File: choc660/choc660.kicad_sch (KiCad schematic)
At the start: 144 parts, among them SW1 SW_Push, SW10 SW_Push, SW11 SW_Push, SW12 SW_Push, SW13 SW_Push, SW14 SW_Push, SW15 SW_Push, SW16 SW_Push, SW17 SW_Push, SW18 SW_Push, SW19 SW_Push, SW2 SW_Push, SW20 SW_Push, SW21 SW_Push, SW22 SW_Push, SW23 SW_Push, SW24 SW_Push, SW25 SW_Push, SW26 SW_Push, SW27 SW_Push, SW28 SW_Push, SW29 SW_Push, SW3 SW_Push, SW30 SW_Push, SW31 SW_Push, SW32 SW_Push, SW33 SW_Push, SW34 SW_Push, SW35 SW_Push, SW36 SW_Push, SW37 SW_Push, SW38 SW_Push, SW39 SW_Push, SW4 SW_Push, SW40 SW_Push, SW41 SW_Push, SW42 SW_Push, SW43 SW_Push, SW44 SW_Push, SW45 SW_Push, SW46 SW_Push, SW47 SW_Push, SW48 SW_Push, SW49 SW_Push, SW5 SW_Push, SW50 SW_Push, SW51 SW_Push, SW52 SW_Push, SW53 SW_Push, SW54 SW_Push, SW55 SW_Push, SW56 SW_Push, SW57 SW_Push, SW58 SW_Push, SW59 SW_Push, SW6 SW_Push, SW60 SW_Push, SW61 SW_Push, SW62 SW_Push, SW63 SW_Push, SW64 SW_Push, SW65 SW_Push, SW66 SW_Push, SW67 SW_Push, SW68 SW_Push, SW7 SW_Push, SW8 SW_Push, SW9 SW_Push, U1 Elite-C

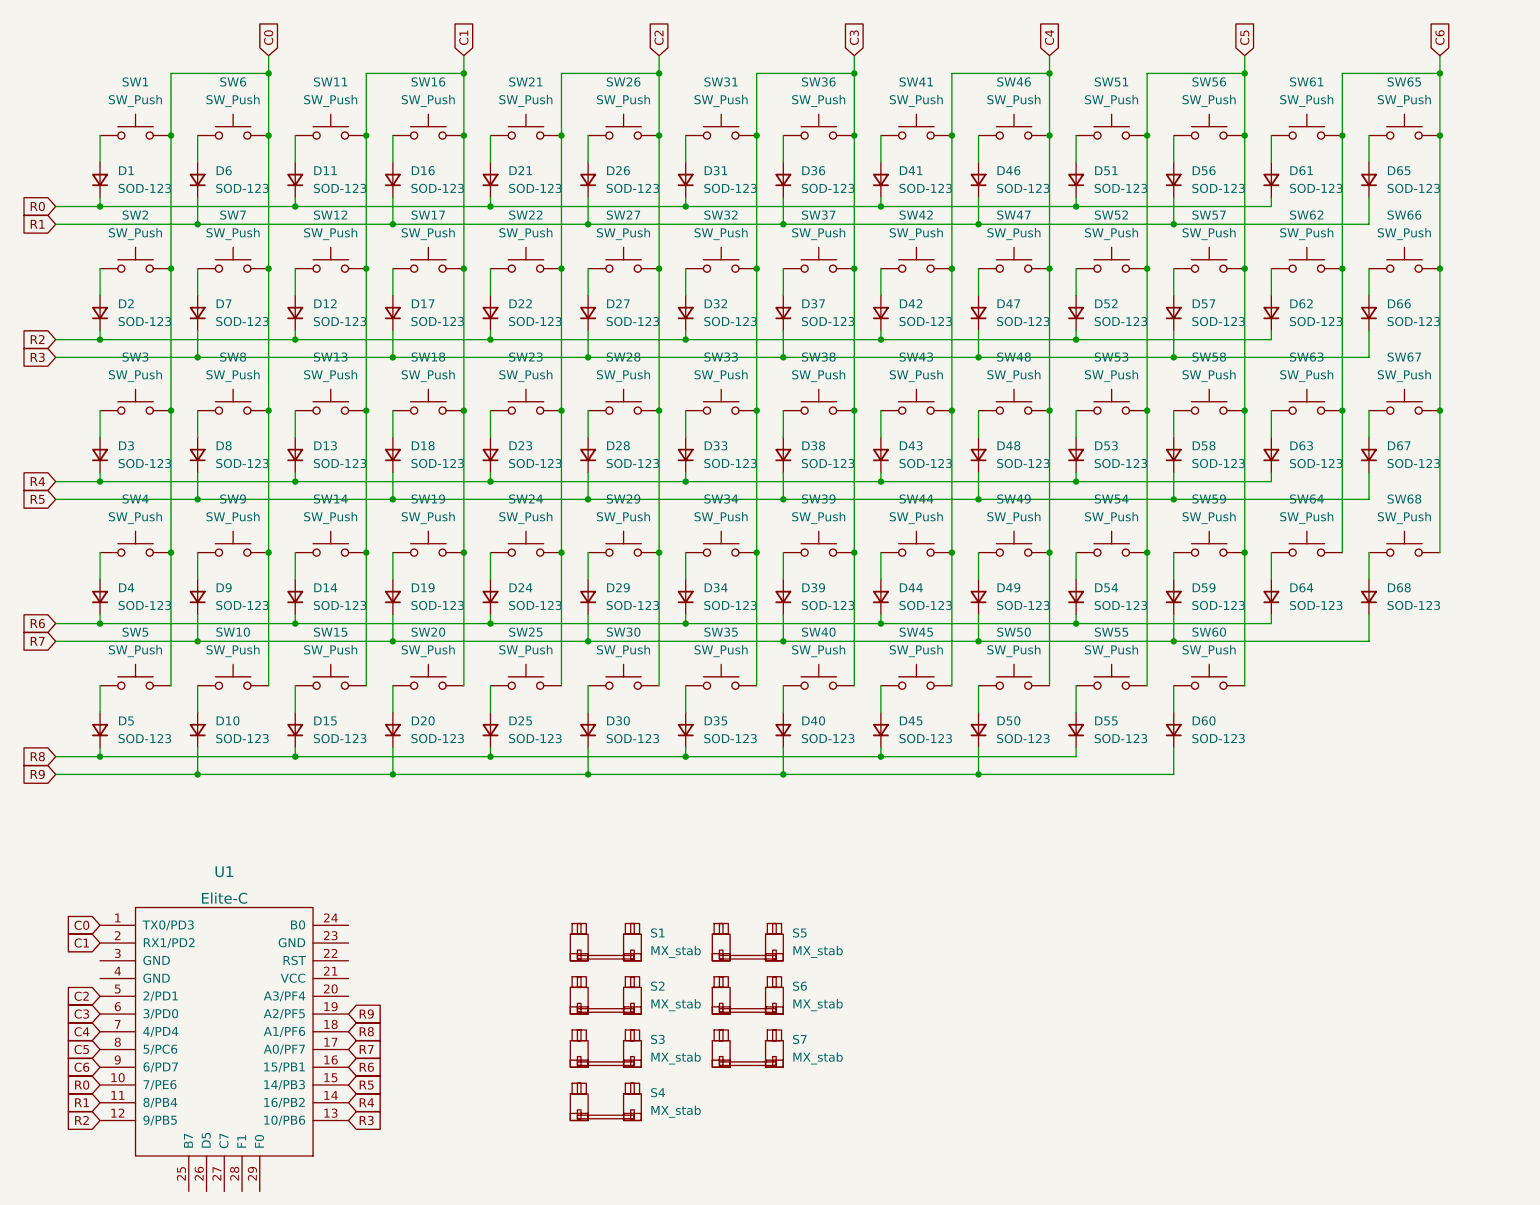
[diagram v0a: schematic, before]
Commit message: draw the rest of the owl?
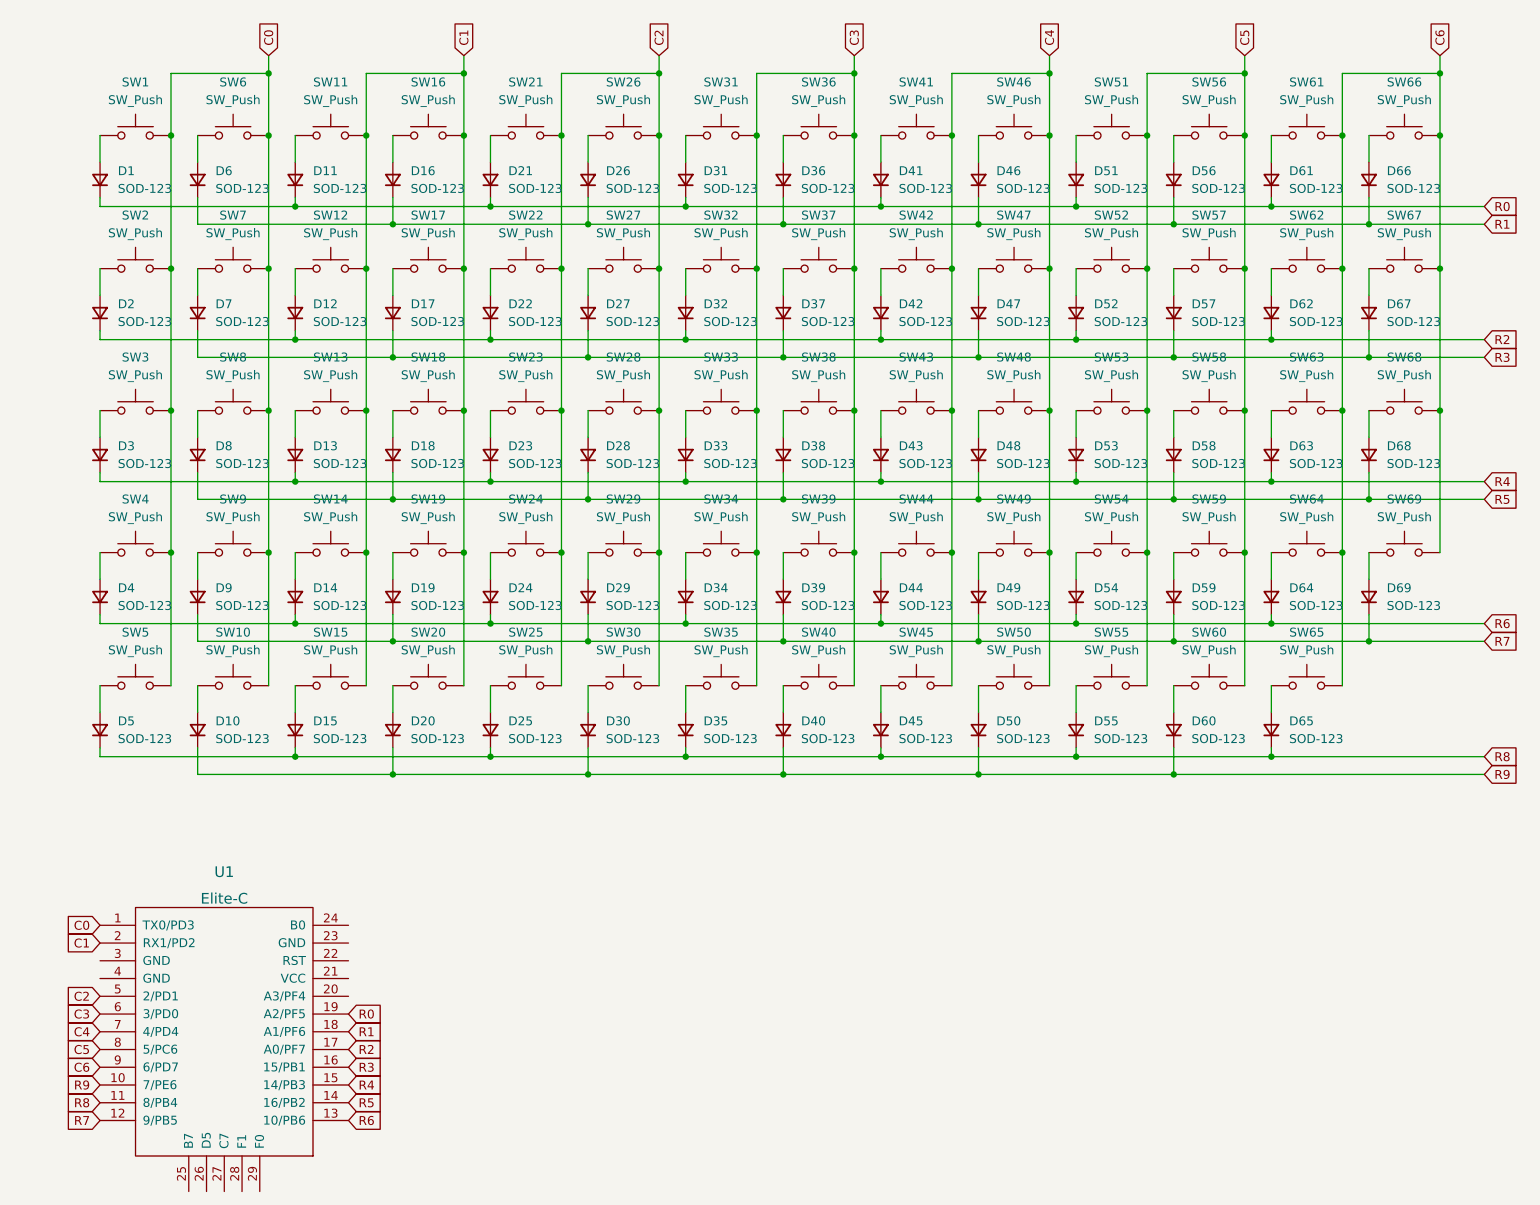
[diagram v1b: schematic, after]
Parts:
- removed S1, S2, S3, S4, S5, S6, S7: MX_stab, marbastlib-choc:STAB_choc_2u, symbol marbastlib-mx:MX_stab
- added D65: SOD-123, Diode_SMD:D_SOD-123, symbol Device:D_Small
- added SW65: SW_Push, marbastlib-choc:SW_choc_HS_1u, symbol Switch:SW_Push
- SW20, SW25, SW30, SW35, SW4, SW59, SW63: footprint marbastlib-choc:SW_choc_HS_1u -> marbastlib-choc:SW_choc_HS_1.5u
- SW66: renamed from SW65; footprint marbastlib-choc:SW_choc_HS_1u -> marbastlib-choc:SW_choc_HS_1.5u
- SW67: renamed from SW66; footprint marbastlib-choc:SW_choc_HS_1.5u -> marbastlib-choc:SW_choc_HS_1u
- renumbered D65 to D66, D66 to D67, D67 to D68, D68 to D69, SW67 to SW68, SW68 to SW69
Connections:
- net C6: now also SW65.2
- net R0: now also U1.19 (A2/PF5); no longer U1.10 (7/PE6)
- net R1: now also U1.18 (A1/PF6); no longer U1.11 (8/PB4)
- net R2: now also U1.17 (A0/PF7); no longer U1.12 (9/PB5)
- net R3: now also U1.16 (15/PB1); no longer U1.13 (10/PB6)
- net R4: now also U1.15 (14/PB3); no longer U1.14 (16/PB2)
- net R5: now also U1.14 (16/PB2); no longer U1.15 (14/PB3)
- net R6: now also U1.13 (10/PB6); no longer U1.16 (15/PB1)
- net R7: now also U1.12 (9/PB5); no longer U1.17 (A0/PF7)
- net R8: now also U1.11 (8/PB4), D65.1 (K); no longer U1.18 (A1/PF6)
- net R9: now also U1.10 (7/PE6); no longer U1.19 (A2/PF5)
- new net: D65.2 (A), SW65.1

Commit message: use non-hotswap footprints, also i made this backwards
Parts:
- SW1, SW10, SW11, SW12, SW13, SW14, SW15, SW16, SW17, SW18, SW19, SW21, SW22, SW23, SW24, SW26, SW27, SW28, SW29, SW31, SW32, SW33, SW34, SW36, SW37, SW38, SW39, SW40, SW41, SW42, SW43, SW44, SW45, SW46, SW47, SW48, SW49, SW5, SW50, SW51, SW52, SW53, SW54, SW55, SW56, SW57, SW58, SW6, SW60, SW61, SW62, SW64, SW65, SW67, SW68, SW69, SW7, SW8, SW9: footprint marbastlib-choc:SW_choc_HS_1u -> marbastlib-choc:SW_choc_1u
- SW2, SW25, SW3, SW30, SW35, SW4, SW59, SW63, SW66: footprint marbastlib-choc:SW_choc_HS_1.5u -> marbastlib-choc:SW_choc_1.5u
- SW20: footprint marbastlib-choc:SW_choc_HS_1.5u -> marbastlib-choc:SW_choc_1.25u

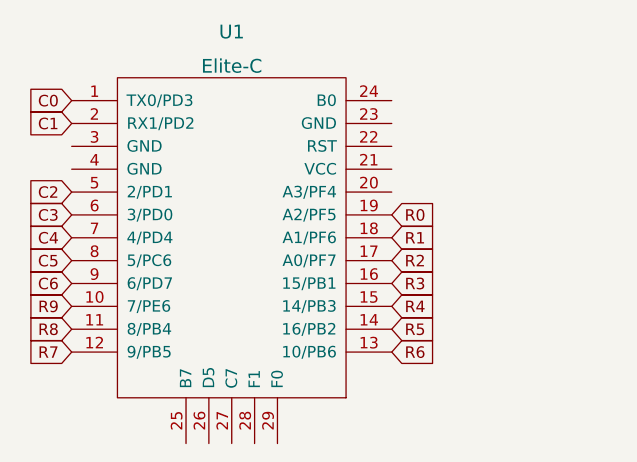
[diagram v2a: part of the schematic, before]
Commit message: retrace, reorient, and all that
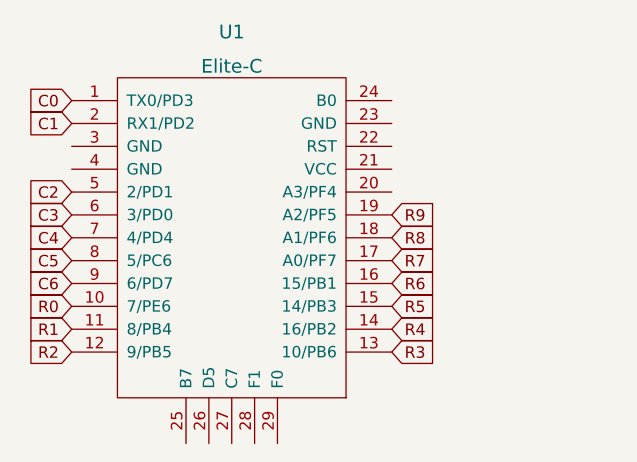
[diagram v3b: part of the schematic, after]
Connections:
- net R0: now also U1.10 (7/PE6); no longer U1.19 (A2/PF5)
- net R1: now also U1.11 (8/PB4); no longer U1.18 (A1/PF6)
- net R2: now also U1.12 (9/PB5); no longer U1.17 (A0/PF7)
- net R3: now also U1.13 (10/PB6); no longer U1.16 (15/PB1)
- net R4: now also U1.14 (16/PB2); no longer U1.15 (14/PB3)
- net R5: now also U1.15 (14/PB3); no longer U1.14 (16/PB2)
- net R6: now also U1.16 (15/PB1); no longer U1.13 (10/PB6)
- net R7: now also U1.17 (A0/PF7); no longer U1.12 (9/PB5)
- net R8: now also U1.18 (A1/PF6); no longer U1.11 (8/PB4)
- net R9: now also U1.19 (A2/PF5); no longer U1.10 (7/PE6)
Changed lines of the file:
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@@
     )
   )
-  (global_label "R5" (shape input) (at 67.31 167.64 0) (fields_autoplaced)
+  (global_label "R4" (shape input) (at 67.31 167.64 0) (fields_autoplaced)
     (effects (font (size 1.27 1.27)) (justify left))
     (property "Intersheet References" "${INTERSHEET_REFS}" (id 0) (at 72.2026 167.5606 0)
@@
     )
   )
-  (global_label "R3" (shape input) (at 67.31 162.56 0) (fields_autoplaced)
+  (global_label "R6" (shape input) (at 67.31 162.56 0) (fields_autoplaced)
     (effects (font (size 1.27 1.27)) (justify left))
     (property "Intersheet References" "${INTERSHEET_REFS}" (id 0) (at 72.2026 162.4806 0)
@@
     )
   )
-  (global_label "R9" (shape input) (at 31.75 165.1 180) (fields_autoplaced)
+  (global_label "R0" (shape input) (at 31.75 165.1 180) (fields_autoplaced)
     (effects (font (size 1.27 1.27)) (justify right))
     (property "Intersheet References" "${INTERSHEET_REFS}" (id 0) (at 26.8574 165.0206 0)
@@
     )
   )
-  (global_label "R6" (shape input) (at 67.31 170.18 0) (fields_autoplaced)
+  (global_label "R3" (shape input) (at 67.31 170.18 0) (fields_autoplaced)
     (effects (font (size 1.27 1.27)) (justify left))
     (property "Intersheet References" "${INTERSHEET_REFS}" (id 0) (at 72.2026 170.1006 0)
@@
     )
   )
-  (global_label "R4" (shape input) (at 67.31 165.1 0) (fields_autoplaced)
+  (global_label "R5" (shape input) (at 67.31 165.1 0) (fields_autoplaced)
     (effects (font (size 1.27 1.27)) (justify left))
     (property "Intersheet References" "${INTERSHEET_REFS}" (id 0) (at 72.2026 165.0206 0)
@@
     )
   )
-  (global_label "R7" (shape input) (at 31.75 170.18 180) (fields_autoplaced)
+  (global_label "R2" (shape input) (at 31.75 170.18 180) (fields_autoplaced)
     (effects (font (size 1.27 1.27)) (justify right))
     (property "Intersheet References" "${INTERSHEET_REFS}" (id 0) (at 26.8574 170.1006 0)
@@
     )
   )
-  (global_label "R0" (shape input) (at 67.31 154.94 0) (fields_autoplaced)
+  (global_label "R9" (shape input) (at 67.31 154.94 0) (fields_autoplaced)
     (effects (font (size 1.27 1.27)) (justify left))
     (property "Intersheet References" "${INTERSHEET_REFS}" (id 0) (at 72.2026 154.8606 0)
@@
     )
   )
-  (global_label "R8" (shape input) (at 31.75 167.64 180) (fields_autoplaced)
+  (global_label "R1" (shape input) (at 31.75 167.64 180) (fields_autoplaced)
     (effects (font (size 1.27 1.27)) (justify right))
     (property "Intersheet References" "${INTERSHEET_REFS}" (id 0) (at 26.8574 167.5606 0)
@@
     )
   )
-  (global_label "R1" (shape input) (at 67.31 157.48 0) (fields_autoplaced)
+  (global_label "R8" (shape input) (at 67.31 157.48 0) (fields_autoplaced)
     (effects (font (size 1.27 1.27)) (justify left))
     (property "Intersheet References" "${INTERSHEET_REFS}" (id 0) (at 72.2026 157.4006 0)
@@
     )
   )
-  (global_label "R2" (shape input) (at 67.31 160.02 0) (fields_autoplaced)
+  (global_label "R7" (shape input) (at 67.31 160.02 0) (fields_autoplaced)
     (effects (font (size 1.27 1.27)) (justify left))
     (property "Intersheet References" "${INTERSHEET_REFS}" (id 0) (at 72.2026 159.9406 0)

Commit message: fix a footprint
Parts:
- SW20: footprint marbastlib-choc:SW_choc_1.25u -> marbastlib-choc:SW_choc_1.5u
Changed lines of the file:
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@@
     (property "Reference" "SW20" (id 0) (at 78.74 100.33 0))
     (property "Value" "SW_Push" (id 1) (at 78.74 102.87 0))
-    (property "Footprint" "marbastlib-choc:SW_choc_1.25u" (id 2) (at 78.74 102.87 0)
+    (property "Footprint" "marbastlib-choc:SW_choc_1.5u" (id 2) (at 78.74 102.87 0)
       (effects (font (size 1.27 1.27)) hide)
     )
@@
     )
     (path "/d14605ea-d48f-44ad-a2d7-845f3728e2f2"
-      (reference "SW20") (unit 1) (value "SW_Push") (footprint "marbastlib-choc:SW_choc_1.25u")
+      (reference "SW20") (unit 1) (value "SW_Push") (footprint "marbastlib-choc:SW_choc_1.5u")
     )
     (path "/769ec98f-af4d-4aaf-9ae9-776c0dad85f5"
